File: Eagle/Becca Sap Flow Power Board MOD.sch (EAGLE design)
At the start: 40 parts, among them J1 1935161, J2 1935200, U1 V_REG_317SMD, U2 V_REG_317SMD, U3 V_REG_317SMD

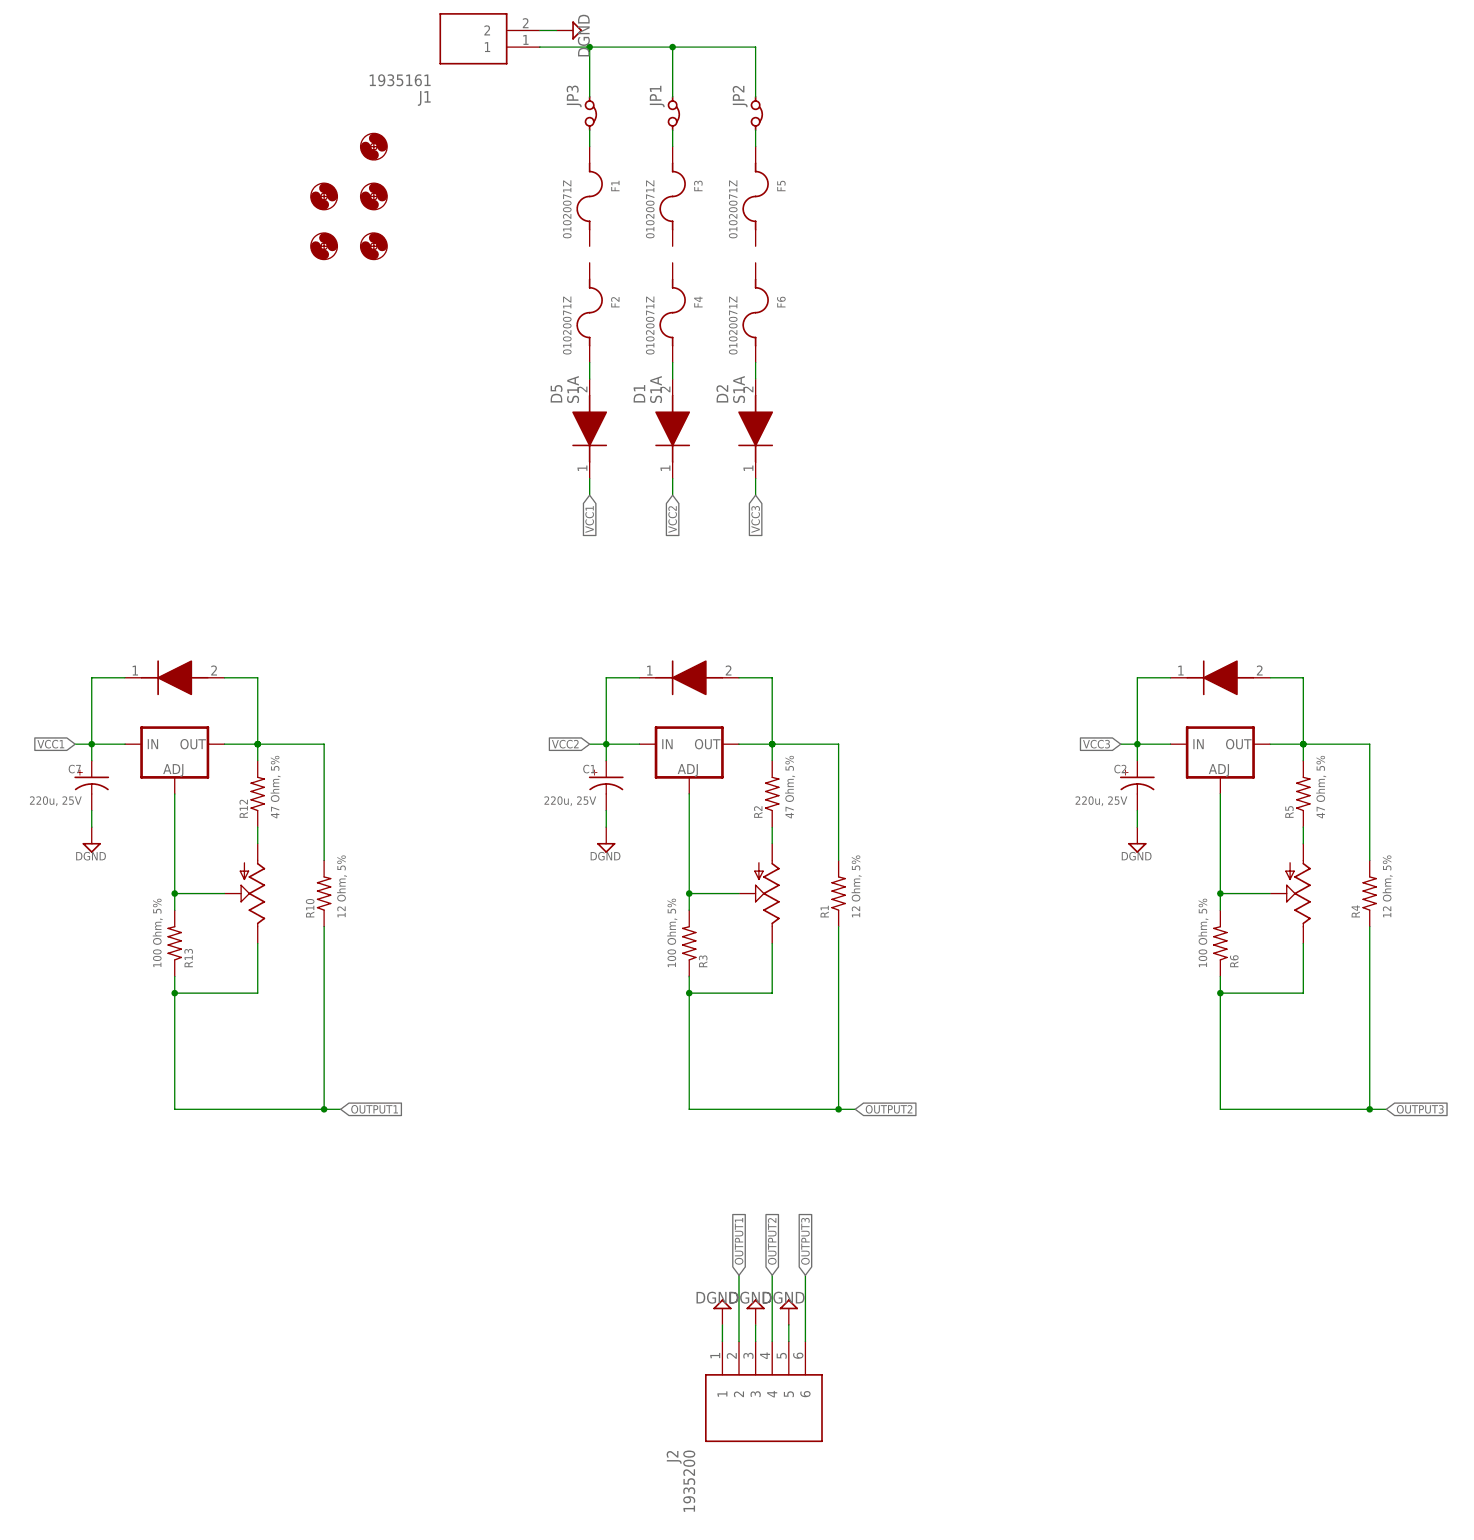
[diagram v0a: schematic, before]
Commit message: Finished boards, generated gerbers and BOM
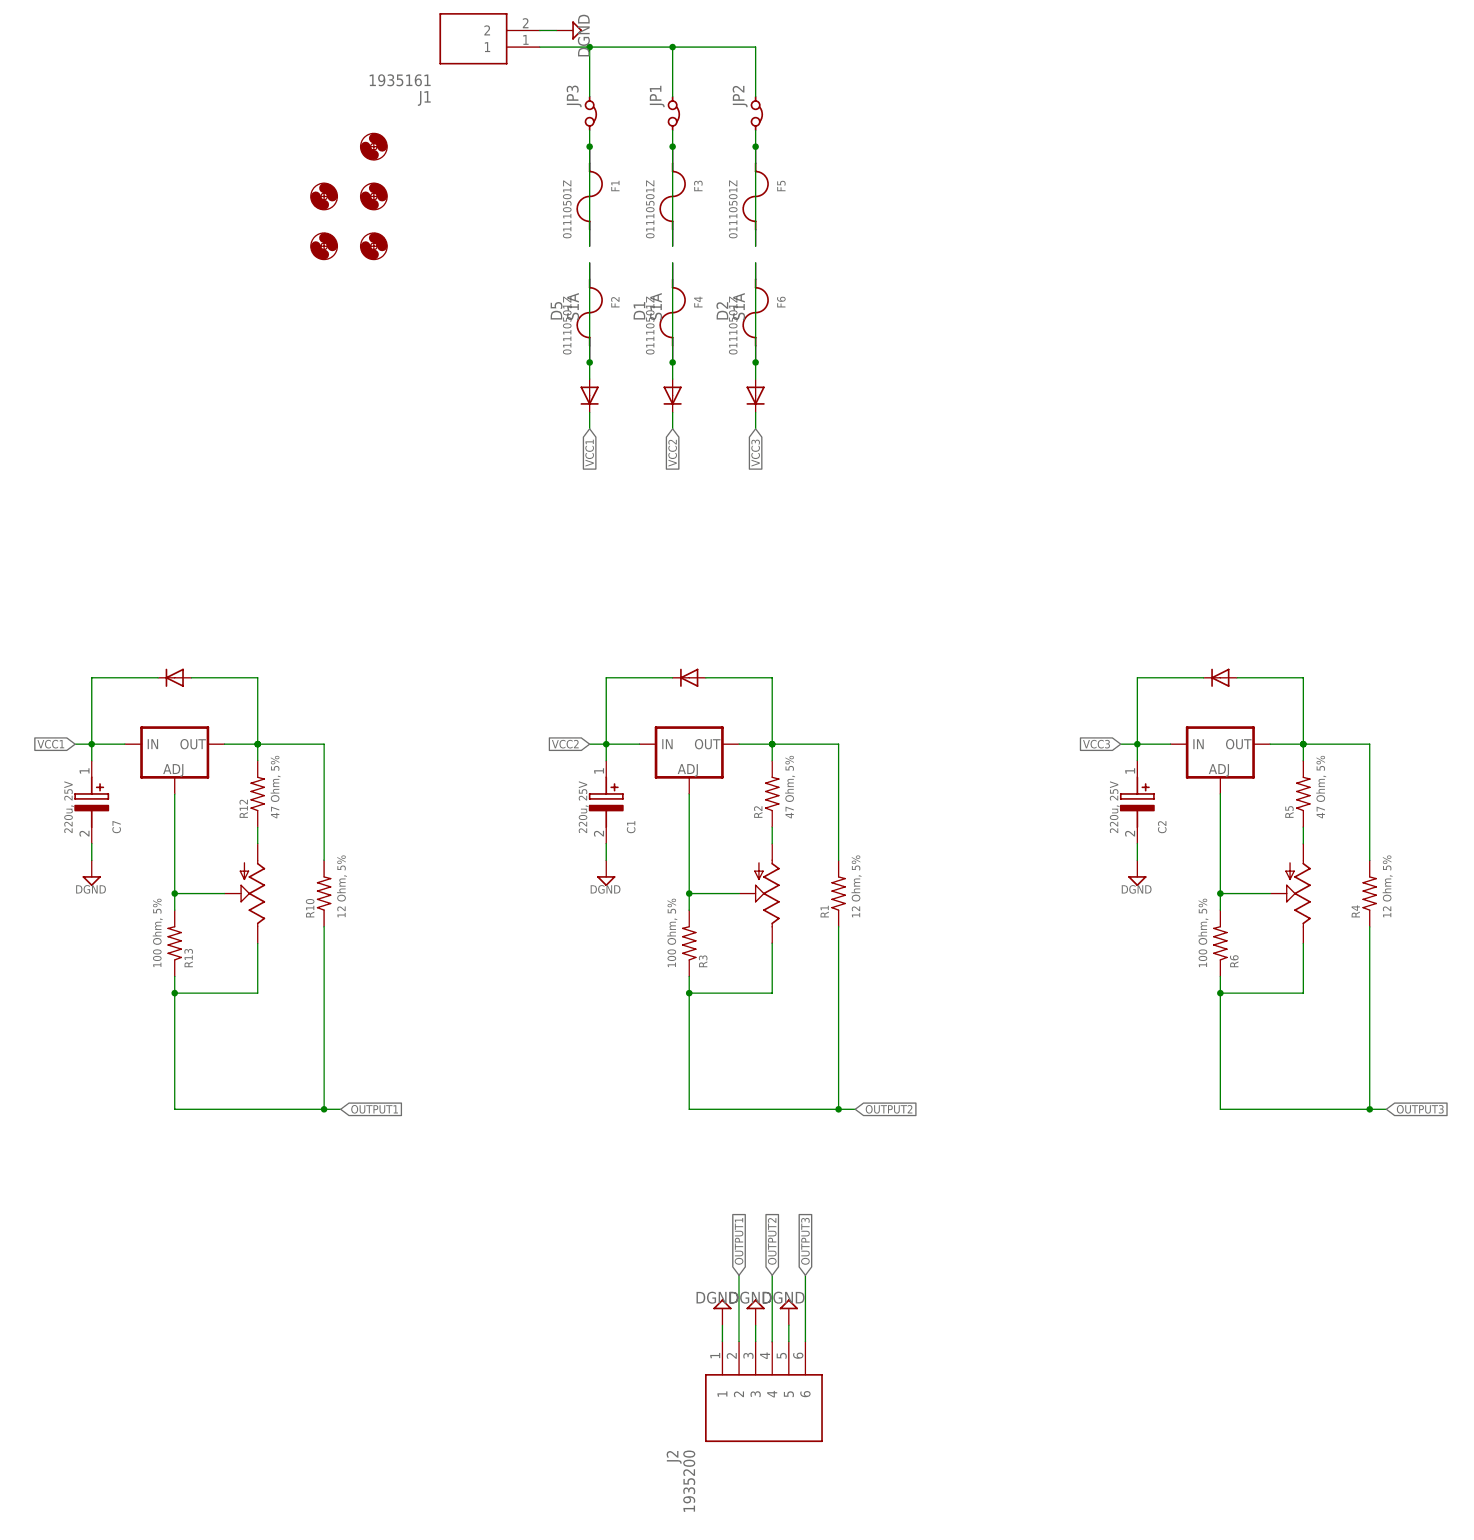
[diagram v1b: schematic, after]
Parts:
- C1, C2, C7: device rcl:CPOL-USC -> Becca-Sap-Flow-LORA:UWT1E221MNL1GS
- D1, D2, D3, D4, D5, D6: device S1A:S1A -> Becca-Sap-Flow-LORA:S1A
- F1, F2, F3, F4, F5, F6: value 01020071Z -> 01110501Z; device Becca-Sap-Flow-LORA:01020071Z -> Becca-Sap-Flow-LORA:01110501Z
- R1, R10, R12, R13, R2, R3, R4, R5, R6: device rcl:R-US_R1210 -> Becca-Sap-Flow-LORA:R-US_R1210
- U1, U2, U3: value V_REG_317SMD -> LM317MBSTT3G; device SparkFun-IC-Power:V_REG_317SMD -> Becca-Sap-Flow-LORA:LM317MBSTT3G
- VR1, VR2, VR3: device 3296W-1-102RLF:3296W-1-102RLF -> Becca-Sap-Flow-LORA:3296W-1-102RLF
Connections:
- net GND renamed DGND
- net N$3: now also F1.2
- net N$4: now also F3.2
- net N$5: now also F2.1
- net N$6: now also F4.1
- net N$8: now also F5.2
- net N$9: now also F6.1
